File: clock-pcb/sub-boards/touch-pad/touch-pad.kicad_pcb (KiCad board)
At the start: 2 copper layers, 99 x 60 mm, 6 parts, among them J1 Conn_01x01_Pin, J2 Conn_01x01_Pin, J3 Conn_01x01_Pin, J4 Conn_01x01_Pin, J5 Conn_01x01_Pin, J6 Conn_01x01_Pin

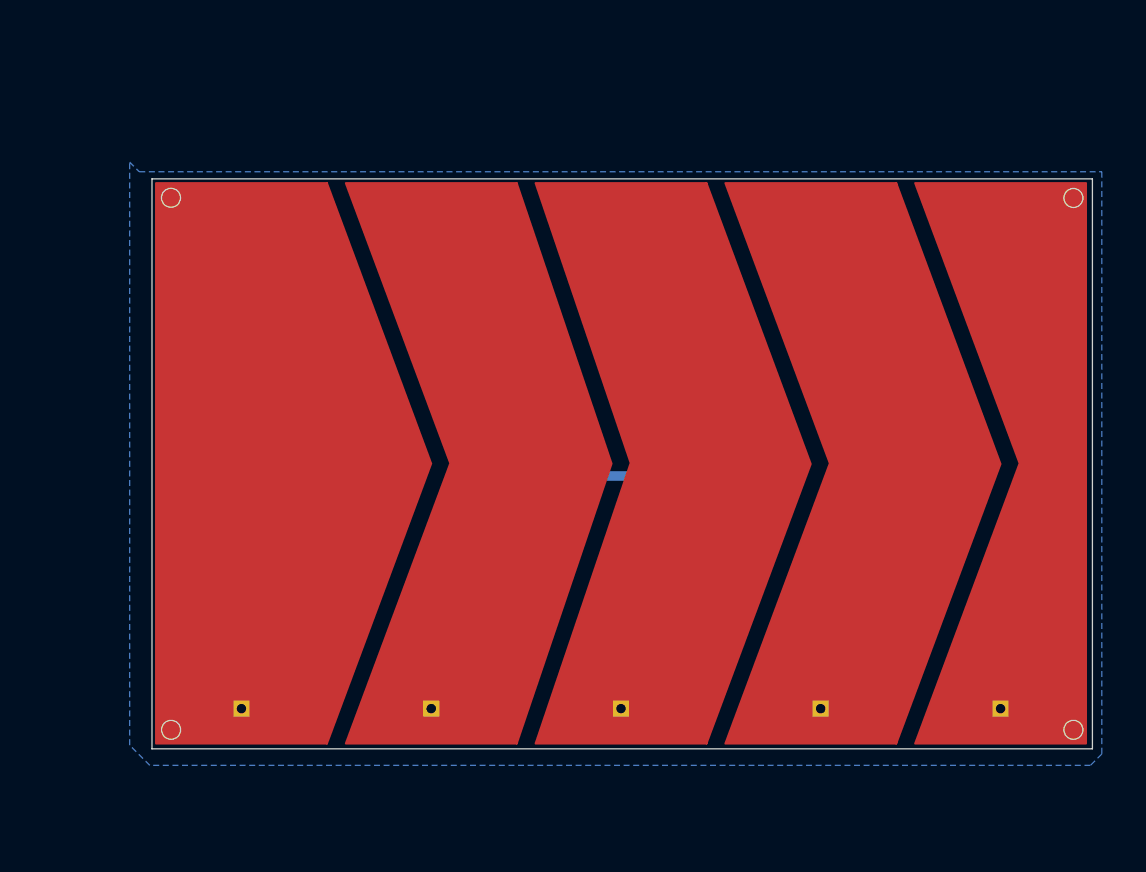
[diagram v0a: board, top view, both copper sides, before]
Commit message: touch slider pcb
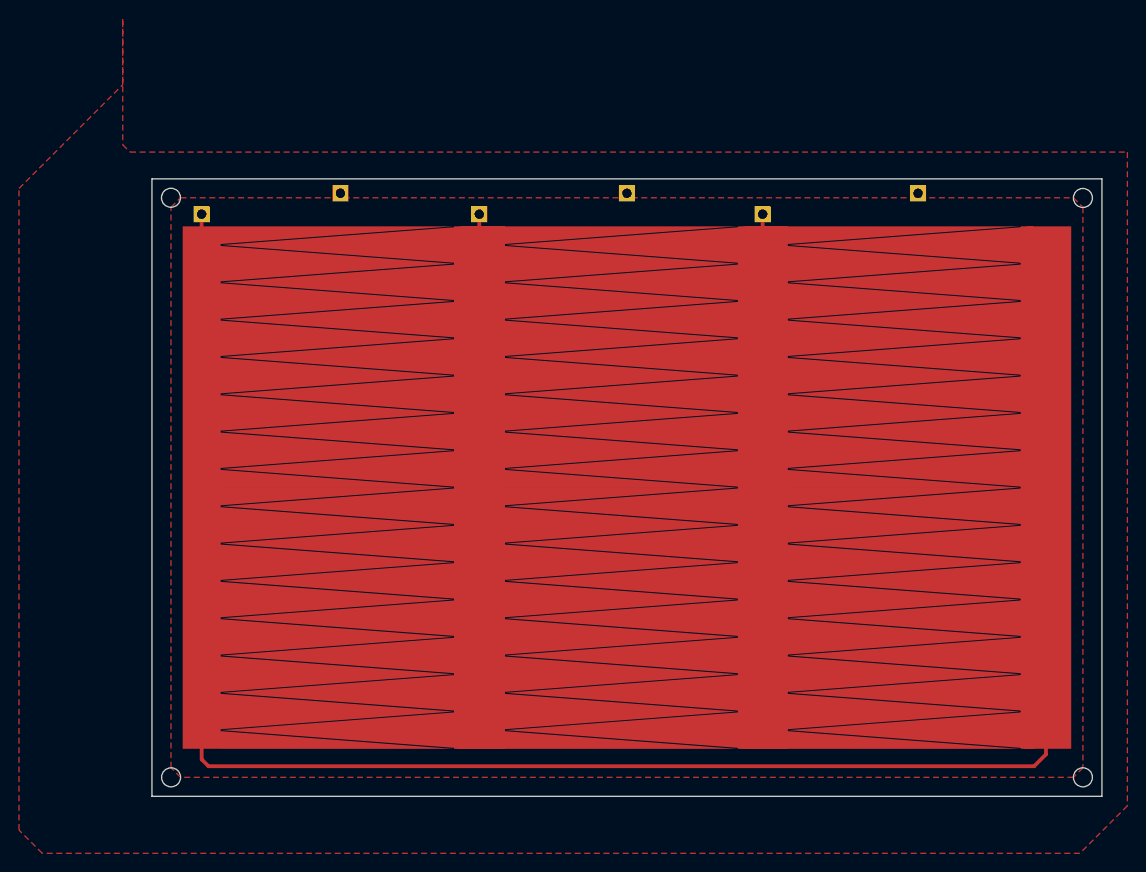
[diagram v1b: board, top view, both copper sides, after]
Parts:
- added J8: Conn_01x04_Pin, clock:TouchSlider-4_90x55mm, F.Cu at (176.3, 99.3)
- J6: footprint Connector_PinHeader_2.54mm:PinHeader_1x02_P2.54mm_Vertical_SMD_Pin1Left -> Connector_PinHeader_2.54mm:PinHeader_1x01_P2.54mm_Vertical
- moved J4 75.6 mm to (160.8, 70.5)
- moved J3 74.6 mm to (207.0, 68.3)
- moved J5 67.7 mm to (176.4, 68.3)
- moved J1 61.8 mm to (146.2, 68.3)
- moved J2 52.4 mm to (190.7, 70.5)
- moved J6 52.3 mm to (131.6, 70.5)
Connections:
- net GPIO2 renamed GUARD
- J1 pad 1: GPIO4_T -> GND
- J2 pad 1: GPIO33 -> SLID_1
- J3 pad 1: GPIO32 -> GND
- J4 pad 1: GPIO27 -> SLID_0
- J6 pad 1: GND -> SLID_2
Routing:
- net SLID_2: track 0.00 -> 175.2 mm
- net SLID_1: track 0.00 -> 29.0 mm
- net SLID_0: track 0.00 -> 28.8 mm
- added copper zone on F.Cu, net GND
- added copper zone on F.Cu, net GUARD
- removed copper zone on B.Cu, net GND
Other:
- board size 99 x 60 mm -> 100 x 65 mm
